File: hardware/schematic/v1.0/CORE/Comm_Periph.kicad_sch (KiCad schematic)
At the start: 20 parts, among them J1 Conn_01x06_Socket, J11 Conn_01x06_Socket, J13 Conn_01x04_Socket, J14 Conn_01x03_Socket, J15 Conn_01x05_Socket, J16 Conn_01x04_Socket

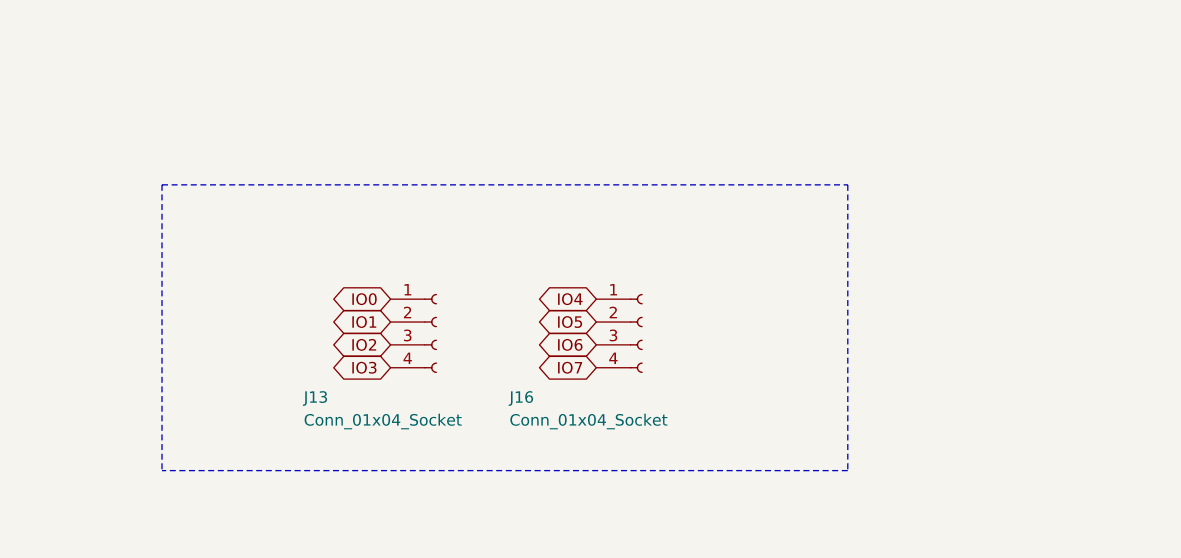
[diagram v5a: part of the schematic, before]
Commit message: sch update
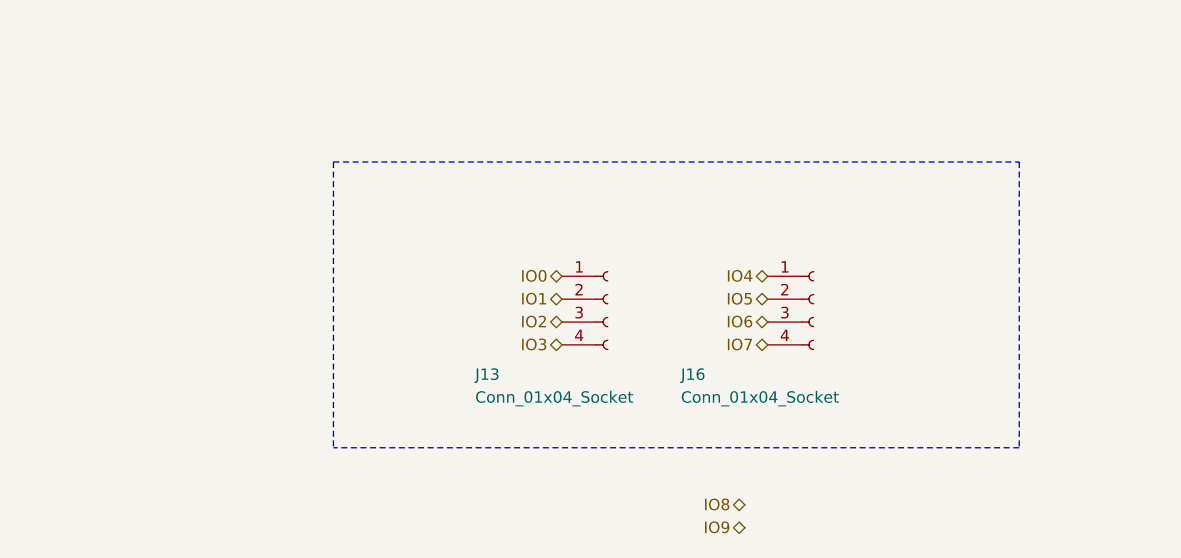
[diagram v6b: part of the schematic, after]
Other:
- moved on the sheet: J13, J16
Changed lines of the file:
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@@
 	(polyline
 		(pts
-			(xy 68.58 125.73) (xy 68.58 157.48)
+			(xy 87.63 123.19) (xy 87.63 154.94)
 		)
 		(stroke
@@
 	(polyline
 		(pts
-			(xy 144.78 125.73) (xy 144.78 157.48)
+			(xy 163.83 123.19) (xy 163.83 154.94)
 		)
 		(stroke
@@
 	(polyline
 		(pts
-			(xy 68.58 125.73) (xy 144.78 125.73)
+			(xy 87.63 123.19) (xy 163.83 123.19)
 		)
 		(stroke
@@
 	(polyline
 		(pts
-			(xy 144.78 157.48) (xy 68.58 157.48)
+			(xy 163.83 154.94) (xy 87.63 154.94)
 		)
 		(stroke
@@
 		)
 	)
-	(global_label "IO6"
+	(hierarchical_label "IO4"
 		(shape bidirectional)
-		(at 116.84 143.51 180)
-		(fields_autoplaced yes)
+		(at 135.89 135.89 180)
 		(effects
 			(font
@@
 			(justify right)
 		)
-		(property "Intersheetrefs" "${INTERSHEET_REFS}"
-			(at 109.5987 143.51 0)
-			(hide yes)
-			(show_name no)
-			(do_not_autoplace no)
-			(effects
-				(font
-					(size 1.27 1.27)
-				)
-				(justify right)
-			)
-		)
 	)
-	(global_label "IO2"
+	(hierarchical_label "IO0"
 		(shape bidirectional)
-		(at 93.98 143.51 180)
-		(fields_autoplaced yes)
+		(at 113.03 135.89 180)
 		(effects
 			(font
@@
 			(justify right)
 		)
-		(property "Intersheetrefs" "${INTERSHEET_REFS}"
-			(at 86.7387 143.51 0)
-			(hide yes)
-			(show_name no)
-			(do_not_autoplace no)
-			(effects
-				(font
-					(size 1.27 1.27)
-				)
-				(justify right)
-			)
-		)
 	)
-	(global_label "IO5"
-		(shape bidirectional)
-		(at 116.84 140.97 180)
-		(fields_autoplaced yes)
-		(effects
-			(font
-				(size 1.27 1.27)
-			)
-			(justify right)
-		)
-		(property "Intersheetrefs" "${INTERSHEET_REFS}"
-			(at 109.5987 140.97 0)
-			(hide yes)
-			(show_name no)
-			(do_not_autoplace no)
-			(effects
-				(font
-					(size 1.27 1.27)
-				)
-				(justify right)
-			)
-		)
-	)
-	(global_label "IO3"
-		(shape bidirectional)
-		(at 93.98 146.05 180)
-		(fields_autoplaced yes)
-		(effects
-			(font
-				(size 1.27 1.27)
-			)
-			(justify right)
-		)
-		(property "Intersheetrefs" "${INTERSHEET_REFS}"
-			(at 86.7387 146.05 0)
-			(hide yes)
-			(show_name no)
-			(do_not_autoplace no)
-			(effects
-				(font
-					(size 1.27 1.27)
-				)
-				(justify right)
-			)
-		)
-	)
-	(global_label "IO7"
+	(hierarchical_label "PS_I2C_SCL"
 		(shape bidirectional)
-		(at 116.84 146.05 180)
-		(fields_autoplaced yes)
+		(at 204.47 72.39 180)
 		(effects
 			(font
@@
 			(justify right)
 		)
-		(property "Intersheetrefs" "${INTERSHEET_REFS}"
-			(at 109.5987 146.05 0)
-			(hide yes)
-			(show_name no)
-			(do_not_autoplace no)
-			(effects
-				(font
-					(size 1.27 1.27)
-				)
-				(justify right)
-			)
-		)
 	)
-	(global_label "IO4"
-		(shape bidirectional)
-		(at 116.84 138.43 180)
-		(fields_autoplaced yes)
+	(hierarchical_label "PL_LED1"
+		(shape input)
+		(at 205.74 128.27 180)
 		(effects
 			(font
@@
 			(justify right)
 		)
-		(property "Intersheetrefs" "${INTERSHEET_REFS}"
-			(at 109.5987 138.43 0)
-			(hide yes)
-			(show_name no)
-			(do_not_autoplace no)
-			(effects
-				(font
-					(size 1.27 1.27)
-				)
-				(justify right)
-			)
-		)
 	)
-	(global_label "IO1"
+	(hierarchical_label "PHY1_MDI1_P"
 		(shape bidirectional)
-		(at 93.98 140.97 180)
-		(fields_autoplaced yes)
+		(at 52.07 57.15 180)
 		(effects
 			(font
@@
 			(justify right)
 		)
-		(property "Intersheetrefs" "${INTERSHEET_REFS}"
-			(at 86.7387 140.97 0)
-			(hide yes)
-			(show_name no)
-			(do_not_autoplace no)
-			(effects
-				(font
-					(size 1.27 1.27)
-				)
-				(justify right)
-			)
-		)
 	)
-	(global_label "IO0"
+	(hierarchical_label "IO3"
 		(shape bidirectional)
-		(at 93.98 138.43 180)
-		(fields_autoplaced yes)
+		(at 113.03 143.51 180)
 		(effects
 			(font
@@
 			(justify right)
 		)
-		(property "Intersheetrefs" "${INTERSHEET_REFS}"
-			(at 86.7387 138.43 0)
-			(hide yes)
-			(show_name no)
-			(do_not_autoplace no)
-			(effects
-				(font
-					(size 1.27 1.27)
-				)
-				(justify right)
-			)
-		)
 	)
-	(hierarchical_label "PS_I2C_SCL"
+	(hierarchical_label "IO5"
 		(shape bidirectional)
-		(at 204.47 72.39 180)
+		(at 135.89 138.43 180)
 		(effects
 			(font
@@
 		)
 	)
-	(hierarchical_label "PL_LED1"
+	(hierarchical_label "PS_SPI1_SS0"
 		(shape input)
-		(at 205.74 128.27 180)
+		(at 231.14 77.47 180)
 		(effects
 			(font
@@
 		)
 	)
-	(hierarchical_label "PHY1_MDI1_P"
+	(hierarchical_label "IO1"
 		(shape bidirectional)
-		(at 52.07 57.15 180)
-		(effects
-			(font
-				(size 1.27 1.27)
-			)
-			(justify right)
-		)
-	)
-	(hierarchical_label "PS_SPI1_SS0"
-		(shape input)
-		(at 231.14 77.47 180)
+		(at 113.03 138.43 180)
 		(effects
 			(font
@@
 		)
 	)
+	(hierarchical_label "IO8"
+		(shape bidirectional)
+		(at 133.35 161.29 180)
+		(effects
+			(font
+				(size 1.27 1.27)
+			)
+			(justify right)
+		)
+	)
 	(hierarchical_label "PHY1_AD0{slash}LED0"
 		(shape bidirectional)
@@
 		)
 	)
+	(hierarchical_label "IO7"
+		(shape bidirectional)
+		(at 135.89 143.51 180)
+		(effects
+			(font
+				(size 1.27 1.27)
+			)
+			(justify right)
+		)
+	)
+	(hierarchical_label "IO6"
+		(shape bidirectional)
+		(at 135.89 140.97 180)
+		(effects
+			(font
+				(size 1.27 1.27)
+			)
+			(justify right)
+		)
+	)
 	(hierarchical_label "PS_SPI1_MOSI"
 		(shape input)
@@
 		)
 	)
+	(hierarchical_label "IO2"
+		(shape bidirectional)
+		(at 113.03 140.97 180)
+		(effects
+			(font
+				(size 1.27 1.27)
+			)
+			(justify right)
+		)
+	)
+	(hierarchical_label "IO9"
+		(shape bidirectional)
+		(at 133.35 163.83 180)
+		(effects
+			(font
+				(size 1.27 1.27)
+			)
+			(justify right)
+		)
+	)
 	(hierarchical_label "PHY1_MDI2_P"
 		(shape bidirectional)
@@
 	(symbol
 		(lib_id "Connector:Conn_01x04_Socket")
-		(at 99.06 140.97 0)
+		(at 118.11 138.43 0)
 		(unit 1)
 		(body_style 1)
@@
 		(dnp no)
 		(property "Reference" "J13"
-			(at 84.328 149.352 0)
+			(at 103.378 146.812 0)
 			(show_name no)
 			(do_not_autoplace no)
@@
 		)
 		(property "Value" "Conn_01x04_Socket"
-			(at 84.328 151.892 0)
+			(at 103.378 149.352 0)
 			(show_name no)
 			(do_not_autoplace no)
@@
 		)
 		(property "Footprint" "Connector_PinHeader_2.54mm:PinHeader_1x04_P2.54mm_Vertical"
-			(at 99.06 140.97 0)
+			(at 118.11 138.43 0)
 			(hide yes)
 			(show_name no)
@@
 		)
 		(property "Datasheet" ""
-			(at 99.06 140.97 0)
+			(at 118.11 138.43 0)
 			(hide yes)
 			(show_name no)
@@
 		)
 		(property "Description" "Generic connector, single row, 01x04, script generated"
-			(at 99.06 140.97 0)
+			(at 118.11 138.43 0)
 			(hide yes)
 			(show_name no)
@@
 	(symbol
 		(lib_id "Connector:Conn_01x04_Socket")
-		(at 121.92 140.97 0)
+		(at 140.97 138.43 0)
 		(unit 1)
 		(body_style 1)
@@
 		(dnp no)
 		(property "Reference" "J16"
-			(at 107.188 149.352 0)
+			(at 126.238 146.812 0)
 			(show_name no)
 			(do_not_autoplace no)
@@
 		)
 		(property "Value" "Conn_01x04_Socket"
-			(at 107.188 151.892 0)
+			(at 126.238 149.352 0)
 			(show_name no)
 			(do_not_autoplace no)
@@
 		)
 		(property "Footprint" "Connector_PinHeader_2.54mm:PinHeader_1x04_P2.54mm_Vertical"
-			(at 121.92 140.97 0)
+			(at 140.97 138.43 0)
 			(hide yes)
 			(show_name no)
@@
 		)
 		(property "Datasheet" ""
-			(at 121.92 140.97 0)
+			(at 140.97 138.43 0)
 			(hide yes)
 			(show_name no)
@@
 		)
 		(property "Description" "Generic connector, single row, 01x04, script generated"
-			(at 121.92 140.97 0)
+			(at 140.97 138.43 0)
 			(hide yes)
 			(show_name no)
